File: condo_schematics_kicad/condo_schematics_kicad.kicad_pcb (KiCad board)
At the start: 2 copper layers, 40.6 x 30.5 mm, 3 parts, among them J1 Conn_01x02_Male

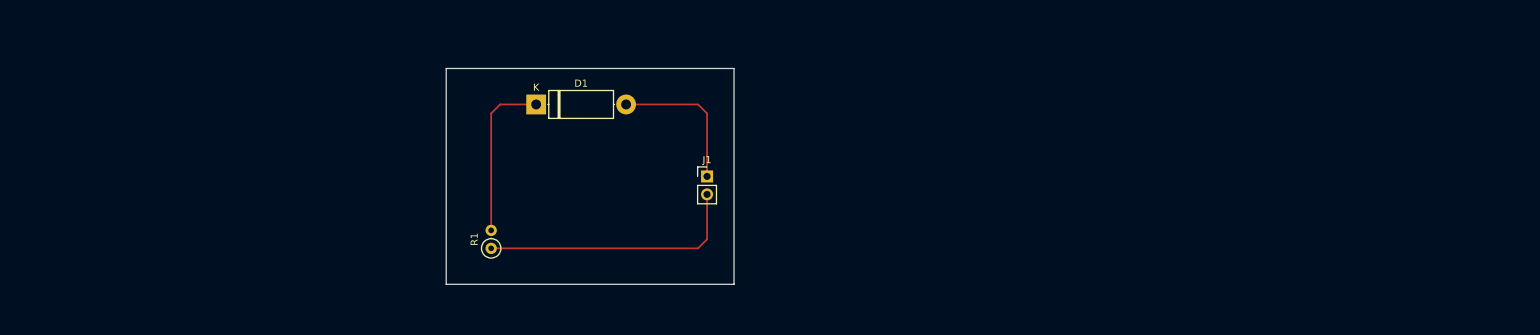
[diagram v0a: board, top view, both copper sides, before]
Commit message: Adding kicad schematics and PCB
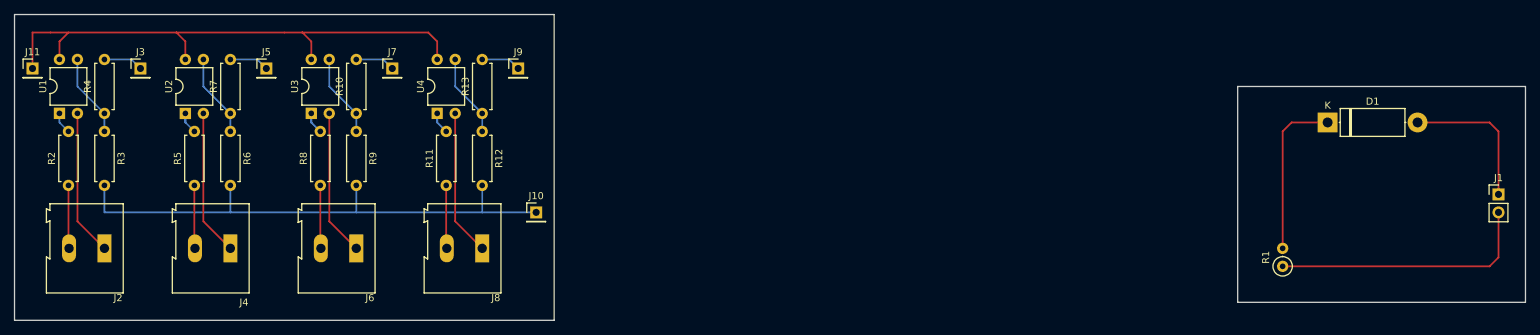
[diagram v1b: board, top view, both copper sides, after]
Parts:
- added J10: Conn_01x01_Male, Connector_PinHeader_2.54mm:PinHeader_1x01_P2.54mm_Vertical, F.Cu at (132.1, 109.2)
- added J11: Conn_01x01_Male, Connector_PinHeader_2.54mm:PinHeader_1x01_P2.54mm_Vertical, F.Cu at (61.0, 88.9)
- added J2: Screw_Terminal_01x02, TerminalBlock:TerminalBlock_Altech_AK300-2_P5.00mm, F.Cu at (71.1, 114.3)
- added J3: Conn_01x01_Male, Connector_PinHeader_2.54mm:PinHeader_1x01_P2.54mm_Vertical, F.Cu at (76.2, 88.9)
- added J4: Screw_Terminal_01x02, TerminalBlock:TerminalBlock_Altech_AK300-2_P5.00mm, F.Cu at (88.9, 114.3)
- added J5: Conn_01x01_Male, Connector_PinHeader_2.54mm:PinHeader_1x01_P2.54mm_Vertical, F.Cu at (94.0, 88.9)
- added J6: Screw_Terminal_01x02, TerminalBlock:TerminalBlock_Altech_AK300-2_P5.00mm, F.Cu at (106.7, 114.3)
- added J7: Conn_01x01_Male, Connector_PinHeader_2.54mm:PinHeader_1x01_P2.54mm_Vertical, F.Cu at (111.8, 88.9)
- added J8: Screw_Terminal_01x02, TerminalBlock:TerminalBlock_Altech_AK300-2_P5.00mm, F.Cu at (124.5, 114.3)
- added J9: Conn_01x01_Male, Connector_PinHeader_2.54mm:PinHeader_1x01_P2.54mm_Vertical, F.Cu at (129.5, 88.9)
- added R10: R, Resistor_THT:R_Axial_DIN0207_L6.3mm_D2.5mm_P7.62mm_Horizontal, F.Cu at (106.7, 95.2)
- added R11: 110, Resistor_THT:R_Axial_DIN0207_L6.3mm_D2.5mm_P7.62mm_Horizontal, F.Cu at (119.4, 105.4)
- added R12: R, Resistor_THT:R_Axial_DIN0207_L6.3mm_D2.5mm_P7.62mm_Horizontal, F.Cu at (124.5, 97.8)
- added R13: R, Resistor_THT:R_Axial_DIN0207_L6.3mm_D2.5mm_P7.62mm_Horizontal, F.Cu at (124.5, 95.2)
- added R2: 110, Resistor_THT:R_Axial_DIN0207_L6.3mm_D2.5mm_P7.62mm_Horizontal, F.Cu at (66.0, 105.4)
- added R3: R, Resistor_THT:R_Axial_DIN0207_L6.3mm_D2.5mm_P7.62mm_Horizontal, F.Cu at (71.1, 97.8)
- added R4: R, Resistor_THT:R_Axial_DIN0207_L6.3mm_D2.5mm_P7.62mm_Horizontal, F.Cu at (71.1, 95.2)
- added R5: 110, Resistor_THT:R_Axial_DIN0207_L6.3mm_D2.5mm_P7.62mm_Horizontal, F.Cu at (83.8, 105.4)
- added R6: R, Resistor_THT:R_Axial_DIN0207_L6.3mm_D2.5mm_P7.62mm_Horizontal, F.Cu at (88.9, 97.8)
- added R7: R, Resistor_THT:R_Axial_DIN0207_L6.3mm_D2.5mm_P7.62mm_Horizontal, F.Cu at (88.9, 95.2)
- added R8: 110, Resistor_THT:R_Axial_DIN0207_L6.3mm_D2.5mm_P7.62mm_Horizontal, F.Cu at (101.6, 105.4)
- added R9: R, Resistor_THT:R_Axial_DIN0207_L6.3mm_D2.5mm_P7.62mm_Horizontal, F.Cu at (106.7, 97.8)
- added U1: EL817, Package_DIP:DIP-4_W7.62mm, F.Cu at (64.8, 95.2)
- added U2: EL817, Package_DIP:DIP-4_W7.62mm, F.Cu at (82.5, 95.2)
- added U3: EL817, Package_DIP:DIP-4_W7.62mm, F.Cu at (100.3, 95.2)
- added U4: EL817, Package_DIP:DIP-4_W7.62mm, F.Cu at (118.1, 95.2)
- moved J1 111.8 mm to (268.0, 106.7)
- moved R1 111.8 mm to (237.5, 116.8)
- moved D1 111.8 mm to (243.8, 96.5)
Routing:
- net +3V3: track 0.00 -> 78.3 mm
- net GND: track 0.00 -> 76.2 mm
- net Net-(J6-Pad1): track 0.00 -> 20.6 mm
- net Net-(J8-Pad1): track 0.00 -> 20.6 mm
- net Net-(J2-Pad1): track 0.00 -> 20.6 mm
- net Net-(J4-Pad1): track 0.00 -> 20.6 mm
- net Net-(R10-Pad1): track 0.00 -> 11.8 mm
- net Net-(R3-Pad1): track 0.00 -> 11.8 mm
- net Net-(R12-Pad1): track 0.00 -> 11.8 mm
- net Net-(R6-Pad1): track 0.00 -> 11.7 mm
- net Net-(J6-Pad2): track 0.00 -> 8.92 mm
- net Net-(J4-Pad2): track 0.00 -> 8.92 mm
- net Net-(J8-Pad2): track 0.00 -> 8.92 mm
- net Net-(J2-Pad2): track 0.00 -> 8.92 mm
- net Net-(J9-Pad1): track 0.00 -> 5.61 mm
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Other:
- board size 40.6 x 30.5 mm -> 213.4 x 43.2 mm
